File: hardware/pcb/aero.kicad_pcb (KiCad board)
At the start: 4 copper layers, 41 x 50 mm, 308 parts, among them CON1 USB-MICRO-B, CON2 MMCX_CONN, J1 CORTEX_DBG_CONN, J2 LiPoly_Conn, Q1 BSS138, SW1 SW_PUSH, U1 STM32L151C8, U10 BU4SU69G2, U11 BU4SU69G2, U12 NC7WZ17, U13 u-blox_max-7c/q, U14 MAX2659, U2 nRF8001, U3 2450BM14A0002, U4 ms5611, U5 BMX055, U6 AT45DB321E, U7 BQ24040DSQ, U8 TPS783, U9 TPS61041, Y1 Crystal, Y2 32.768KHz, Y3 16MHz

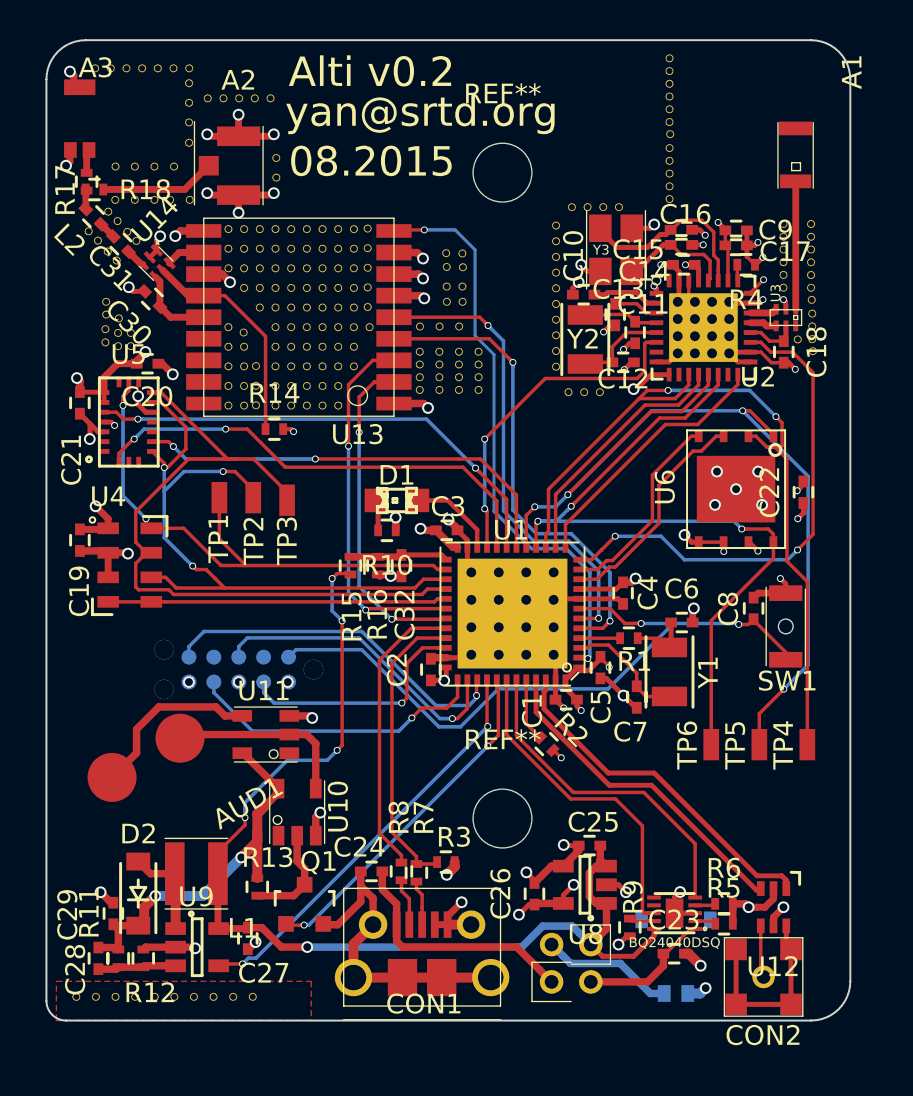
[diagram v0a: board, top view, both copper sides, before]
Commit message: rewired sensors + gps
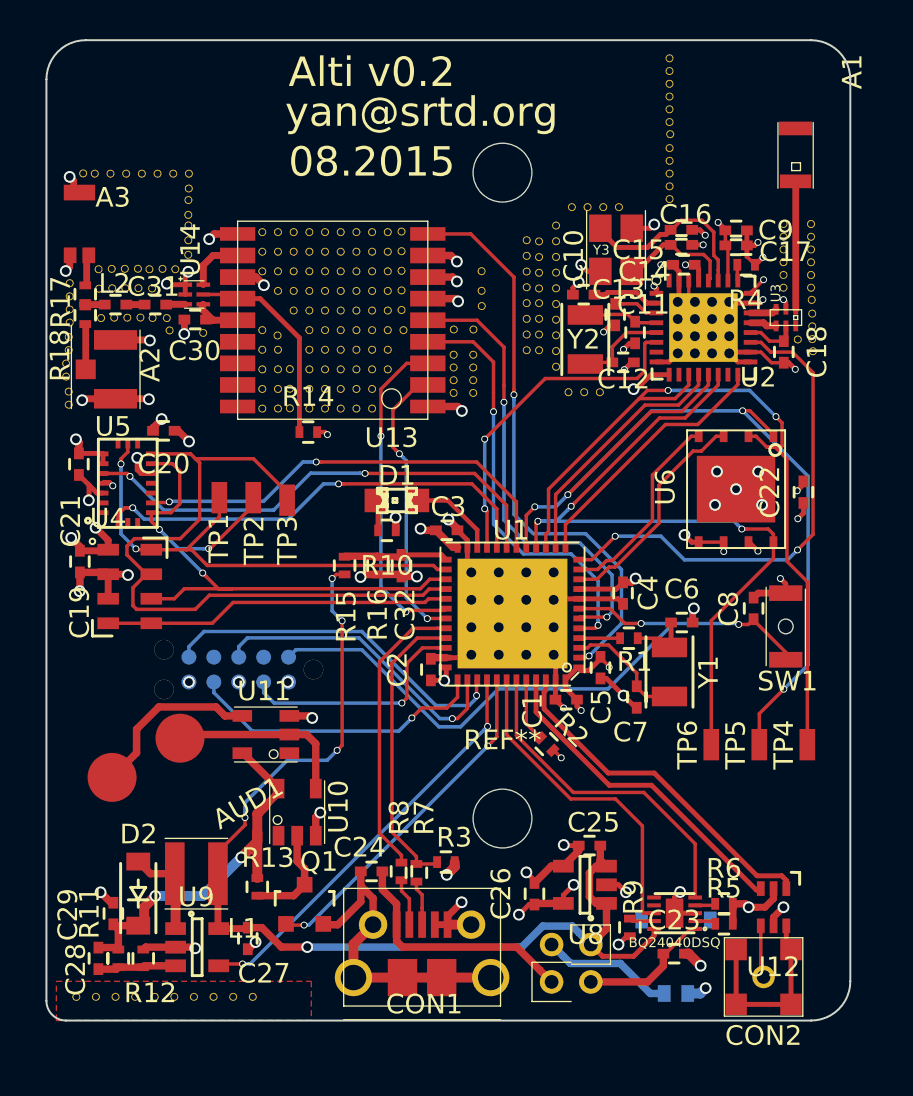
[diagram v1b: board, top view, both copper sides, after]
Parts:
- removed the REF**1111 at (132.3, 68.2)
- removed the REF**1111 at (132.3, 69.2)
- removed the REF**1111 at (132.3, 73.1)
- removed the REF**1111 at (131.3, 73.1)
- removed the REF**1111 at (130.5, 73.1)
- removed the REF**1111 at (129.5, 73.1)
- removed the REF**1111 at (128.5, 73.1)
- removed the REF**1111 at (132.3, 70.2)
- removed the REF**1111 at (136.7, 72.0)
- removed the REF**1111 at (136.7, 71.0)
- removed REF**11111111 (x9), REF**11111112 (x5), REF**11111113 (x3), REF**11731, REF**117311, REF**117312, REF**117313, REF**117314, REF**117411, REF**117412, REF**117413, REF**117414: v, aero:Via_Stitch
- removed the REF**1151 at (133.2, 68.0)
- removed the REF**1161 at (134.0, 68.0)
- removed the REF**1163 at (146.2, 75.9)
- removed the REF**1163 at (146.2, 76.6)
- removed the REF**1171 at (134.8, 68.0)
- removed the REF**1172 at (145.4, 75.9)
- removed the REF**1181 at (135.6, 68.0)
- removed the REF**1183 at (146.2, 77.6)
- removed the REF**1184 at (146.2, 78.3)
- removed the REF**1191 at (136.4, 68.0)
- added REF**1111: v, aero:Via_Stitch, F.Cu at (133.0, 79.9)
- added REF**1111: v, aero:Via_Stitch, F.Cu at (126.1, 80.8)
- added REF**1111: v, aero:Via_Stitch, F.Cu at (126.0, 82.2)
- added REF**1111: v, aero:Via_Stitch, F.Cu at (126.2, 77.4)
- added REF**1111: v, aero:Via_Stitch, F.Cu at (126.2, 78.7)
- added REF**1111: v, aero:Via_Stitch, F.Cu at (126.2, 78.1)
- added REF**1111: v, aero:Via_Stitch, F.Cu at (126.2, 79.4)
- added REF**1111: v, aero:Via_Stitch, F.Cu at (132.2, 75.9)
- added REF**1111: v, aero:Via_Stitch, F.Cu at (132.2, 75.2)
- added REF**1111: v, aero:Via_Stitch, F.Cu at (132.2, 73.9)
- added REF**1111: v, aero:Via_Stitch, F.Cu at (131.6, 76.7)
- added REF**1111: v, aero:Via_Stitch, F.Cu at (131.3, 79.8)
- added REF**1111: v, aero:Via_Stitch, F.Cu at (130.9, 76.7)
- added REF**1111: v, aero:Via_Stitch, F.Cu at (130.3, 76.7)
- added REF**1111: v, aero:Via_Stitch, F.Cu at (129.7, 76.7)
- added REF**1111: v, aero:Via_Stitch, F.Cu at (129.0, 76.7)
- added REF**1111: v, aero:Via_Stitch, F.Cu at (128.3, 76.7)
- added REF**1111: v, aero:Via_Stitch, F.Cu at (127.7, 76.7)
- added REF**1111: v, aero:Via_Stitch, F.Cu at (129.8, 79.1)
- added REF**1111: v, aero:Via_Stitch, F.Cu at (129.1, 79.2)
- added REF**1111: v, aero:Via_Stitch, F.Cu at (127.8, 79.2)
- added REF**1111: v, aero:Via_Stitch, F.Cu at (128.5, 79.2)
- added REF**1111: v, aero:Via_Stitch, F.Cu at (131.1, 79.2)
- added REF**1111: v, aero:Via_Stitch, F.Cu at (130.4, 79.2)
- added REF**1111: v, aero:Via_Stitch, F.Cu at (130.4, 77.7)
- added REF**1111: v, aero:Via_Stitch, F.Cu at (126.1, 83.6)
- added REF**1111: v, aero:Via_Stitch, F.Cu at (126.1, 82.9)
- added REF**1111: v, aero:Via_Stitch, F.Cu at (126.1, 80.1)
- added REF**1111: v, aero:Via_Stitch, F.Cu at (126.0, 81.5)
- added REF**1121: v, aero:Via_Stitch, F.Cu at (126.9, 71.8)
- added REF**117311115: v, aero:Via_Stitch, F.Cu at (149.5, 75.2)
- added REF**117311115: v, aero:Via_Stitch, F.Cu at (149.5, 78.4)
- added REF**117311115: v, aero:Via_Stitch, F.Cu at (150.1, 78.4)
- added REF**117311115: v, aero:Via_Stitch, F.Cu at (150.1, 75.3)
- added REF**117311116: v, aero:Via_Stitch, F.Cu at (149.5, 76.0)
- added REF**117311116: v, aero:Via_Stitch, F.Cu at (149.5, 79.2)
- added REF**117311116: v, aero:Via_Stitch, F.Cu at (150.1, 79.2)
- added REF**117311116: v, aero:Via_Stitch, F.Cu at (150.1, 76.1)
- added REF**117311117: v, aero:Via_Stitch, F.Cu at (149.5, 76.8)
- added REF**117311117: v, aero:Via_Stitch, F.Cu at (149.5, 80.0)
- added REF**117311117: v, aero:Via_Stitch, F.Cu at (150.1, 80.0)
- added REF**117311117: v, aero:Via_Stitch, F.Cu at (150.1, 76.9)
- added REF**117311118: v, aero:Via_Stitch, F.Cu at (149.5, 77.6)
- added REF**117311118: v, aero:Via_Stitch, F.Cu at (149.5, 80.8)
- added REF**117311118: v, aero:Via_Stitch, F.Cu at (150.1, 80.8)
- added REF**117311118: v, aero:Via_Stitch, F.Cu at (150.1, 77.7)
- added REF**1181: v, aero:Via_Stitch, F.Cu at (132.2, 74.4)
- added REF**1181: v, aero:Via_Stitch, F.Cu at (132.2, 73.2)
- moved A2 12.1 mm to (128.5, 81.8)
- moved REF**1111 6.46 mm to (129.7, 77.6)
- moved R18 6.43 mm to (127.0, 79.0), turned to 90 degrees
- moved REF**1111 6.38 mm to (129.0, 77.7)
- moved REF**1111 6.32 mm to (128.4, 77.7)
- moved REF**1111 6.29 mm to (127.7, 77.7)
- moved R17 5.74 mm to (127.0, 78.0)
- moved A3 5.37 mm to (126.7, 74.4)
- moved REF**1111 5.37 mm to (132.3, 72.6)
- moved REF**1121 5.37 mm to (127.5, 71.8)
- moved REF**1131 5.37 mm to (128.3, 71.8)
- moved REF**1141 5.37 mm to (129.1, 71.8)
- moved REF**1151 5.37 mm to (129.9, 71.8)
- moved REF**1161 5.37 mm to (130.7, 71.8)
- moved REF**1171 5.37 mm to (131.5, 71.8)
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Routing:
- net Net-(A2-Pad1): track 5.88 -> 2.32 mm
- net GND: track 129.2 -> 126.0 mm
- net /bmx055/MISO: track 34.8 -> 31.9 mm
- net /GPS/TIMEPULSE: track 24.6 -> 21.9 mm
- net /bmx055/SCK: track 28.1 -> 25.5 mm
- net GPS_TX: track 16.9 -> 14.7 mm
- net Net-(C30-Pad1): track 4.06 -> 2.67 mm
- net GPS_RX: track 18.8 -> 17.7 mm
- net +3V: track 41.6 -> 42.5 mm, vias 25 -> 26
- net Net-(R14-Pad1): track 11.5 -> 10.8 mm
- net /bmx055/MAG_SEL: track 24.1 -> 23.4 mm
- net /GPS/EXT_INT: track 24.5 -> 23.9 mm
- net Net-(A3-Pad1): track 1.32 -> 1.89 mm
